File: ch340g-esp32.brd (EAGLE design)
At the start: 100 x 80 mm, 0 parts

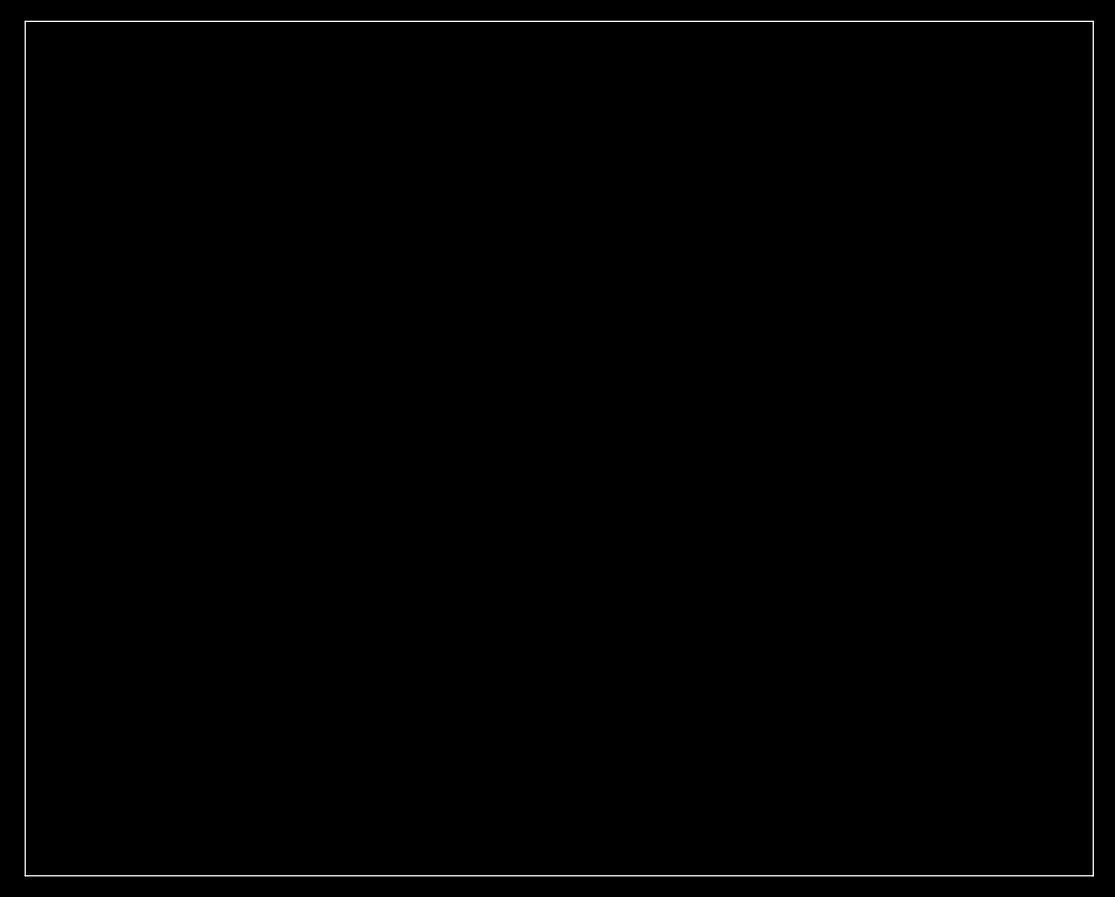
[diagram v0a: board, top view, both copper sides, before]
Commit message: rev1
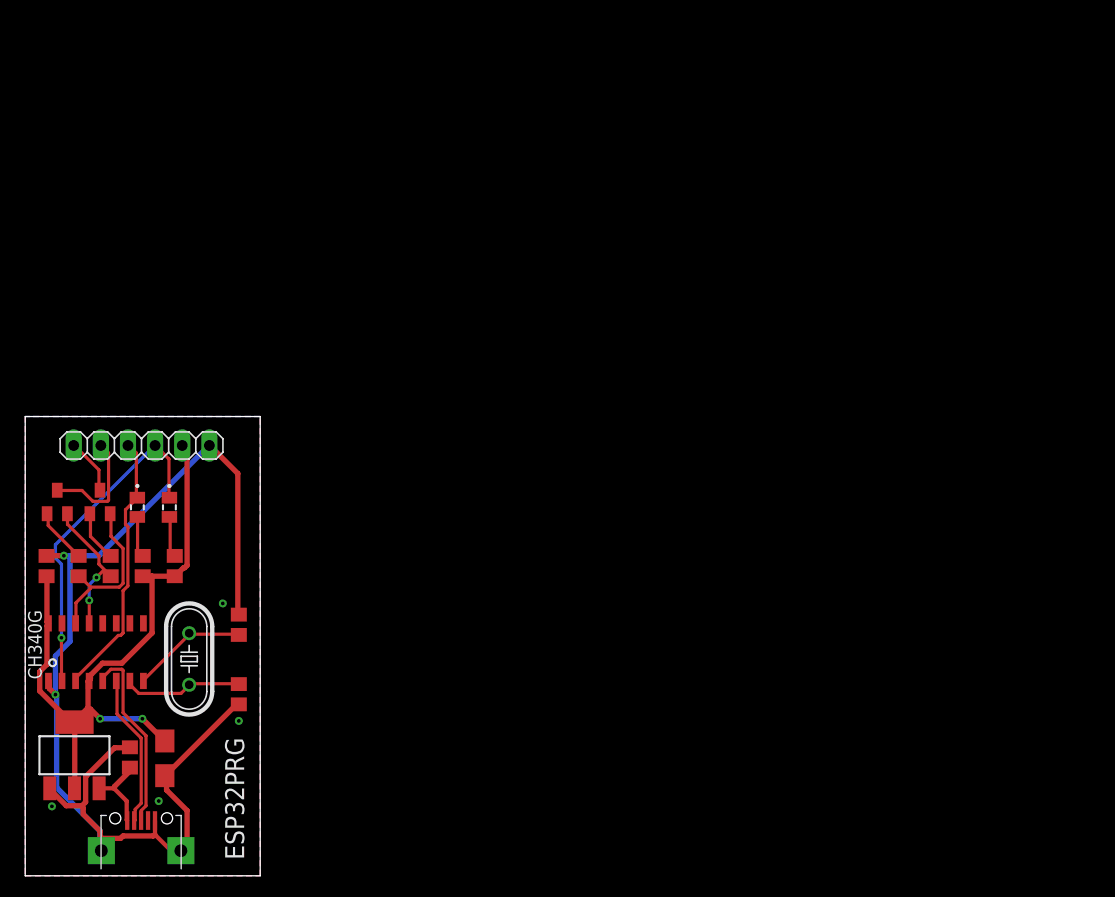
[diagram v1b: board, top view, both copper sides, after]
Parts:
- added C1, C2: 22, rcl:C0805
- added C3, C5: 0.1uF, rcl:C0805
- added C4: 10uF, rcl:B/3528-21W
- added D1: YELLOW, 597-5311-402F:LEDC2012X70N
- added D2: GREEN, 597-5311-402F:LEDC2012X70N
- added IC1: (no value), lm1117:SOT223
- added JP1: OUT, pinhead:1X06
- added Q1: 12M, crystal:HC49/S
- added R1, R2: 10K, rcl:R0805
- added R3, R4: 2K, rcl:R0805
- added T1, T2: BC847, transistor:SOT23
- added U$1: MICRO-USB, microusb:MICRO-USB
- added U$2: CH340G, ch340g:SOIC16
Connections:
- new net +5V: C3.1, IC1.3, U$1.1
- new net D+: U$1.3, U$2.5
- new net D-: U$1.2, U$2.6
- new net DTR: R1.1, T2.2, U$2.13
- new net EN: JP1.1, T1.3
- new net GND: C1.2, C2.2, C3.2, C4.-, C5.2, IC1.1, JP1.6, U$1.5, U$1.GND1, U$1.GND2, U$2.1
- new net IO0: JP1.2, T2.3
- new net N$1: C2.1, Q1.2, U$2.8
- new net N$12: D2.A, R4.1
- new net N$2: C1.1, Q1.1, U$2.7
- new net N$3: R1.2, T1.1
- new net N$4: R2.2, T2.1
- new net N$5: D1.A, R3.1
- new net RTS: R2.1, T1.2, U$2.14
- new net RX: D2.C, JP1.3, U$2.3
- new net TX: D1.C, JP1.4, U$2.2
- new net VCC: C4.+, C5.1, IC1.2, IC1.TAB, JP1.5, R3.2, R4.2, U$2.16, U$2.4
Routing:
- net GND: track 0.00 -> 113.3 mm, vias 0 -> 6
- net VCC: track 0.00 -> 64.0 mm, vias 0 -> 2
- net TX: track 0.00 -> 31.7 mm, vias 0 -> 1
- net RX: track 0.00 -> 25.2 mm
- net D+: track 0.00 -> 17.7 mm
- net RTS: track 0.00 -> 15.7 mm
- net D-: track 0.00 -> 14.4 mm
- net DTR: track 0.00 -> 13.9 mm, vias 0 -> 2
- net N$2: track 0.00 -> 11.3 mm
- net N$1: track 0.00 -> 10.9 mm
- net IO0: track 0.00 -> 10.7 mm
- net +5V: track 0.00 -> 7.46 mm
- net EN: track 0.00 -> 5.25 mm
- net N$4: track 0.00 -> 5.18 mm
- net N$3: track 0.00 -> 4.78 mm
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- added copper zone on layer 1, net GND
- added copper zone on layer 16, net GND
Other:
- board size 100 x 80 mm -> 22 x 43 mm
- board text added: "ESP32PRG"
- board text added: "RST BOOT RX TX 3.3V GND"

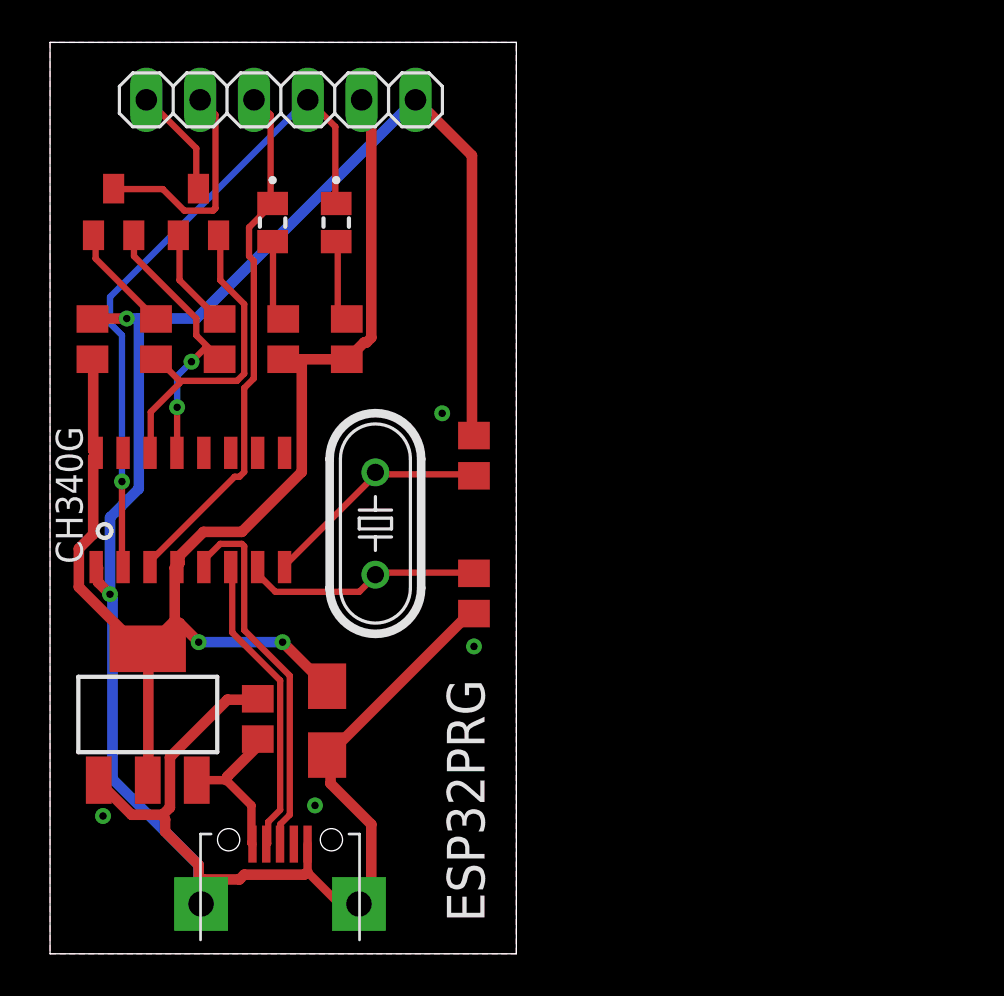
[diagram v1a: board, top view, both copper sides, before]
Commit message: board update
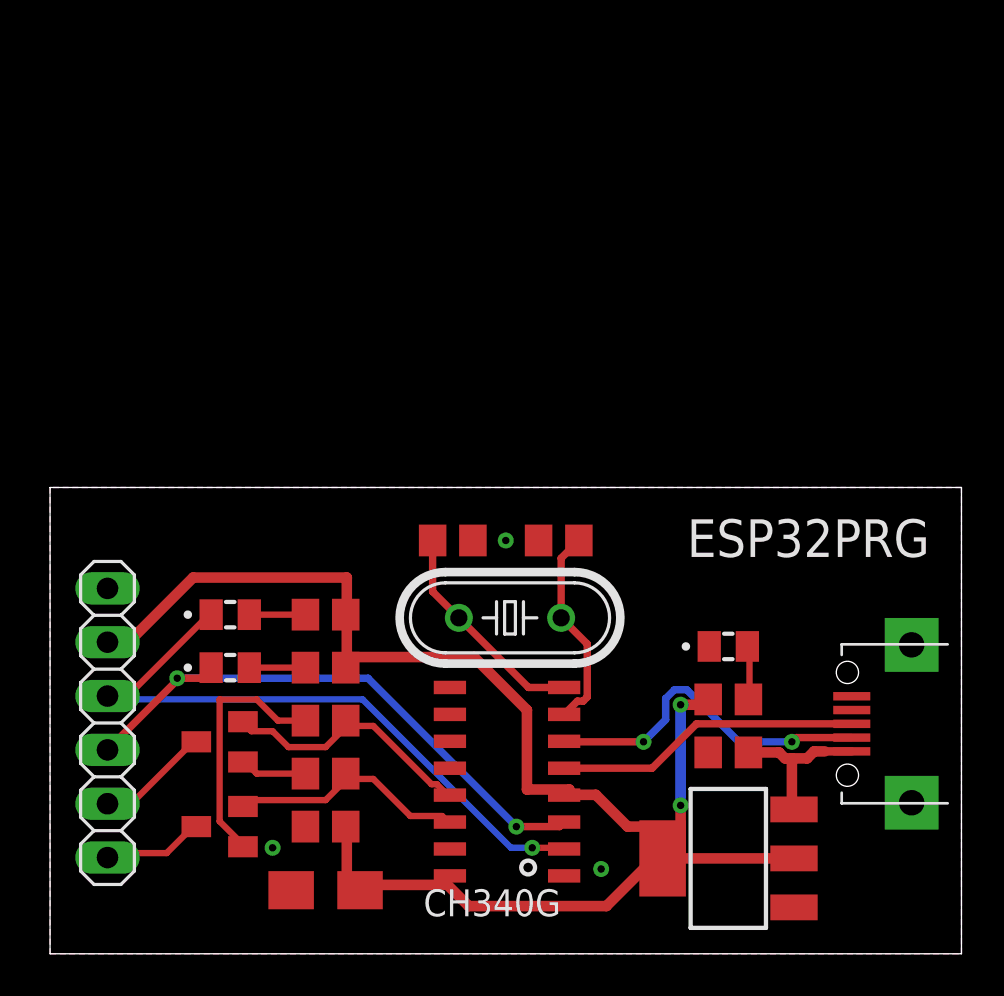
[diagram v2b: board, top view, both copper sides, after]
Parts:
- added D3: GREEN, 597-5311-402F:LEDC2012X70N
- added R5: 2K, rcl:R0805
- moved U$1 33.1 mm to (42.4, 10.8), turned to 90 degrees
- moved JP1 30.5 mm to (2.71, 10.9), turned to 90 degrees
- moved T1 29.0 mm to (8.00, 6.00), turned to 90 degrees
- moved IC1 28.2 mm to (32.0, 4.50), turned to 90 degrees
- moved C5 25.5 mm to (13.0, 6.00), turned to 180 degrees
- moved T2 25.5 mm to (8.00, 10.0), turned to 90 degrees
- moved C3 22.3 mm to (32.0, 9.50), turned to 180 degrees
- moved R2 22.0 mm to (13.0, 8.50), turned to 180 degrees
- moved D2 21.1 mm to (8.50, 13.5), turned to 0 degrees
- moved U$2 19.7 mm to (21.6, 8.12), turned to 90 degrees
- moved D1 19.2 mm to (8.50, 16.0), turned to 0 degrees
- moved R1 18.7 mm to (13.0, 11.0), turned to 180 degrees
- moved R4 15.6 mm to (13.0, 13.5), turned to 0 degrees
- moved R3 13.0 mm to (13.0, 16.0), turned to 0 degrees
- moved C4 8.00 mm to (13.0, 3.00), turned to 0 degrees
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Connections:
- new net N$6: D3.A, R5.1
- net GND: now also D3.C
- net VCC: now also R5.2
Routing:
- net GND: track 113.3 -> 0.00 mm, vias 6 -> 3
- net VCC: track 64.0 -> 76.0 mm
- net N$3: track 4.78 -> 11.9 mm
- net IO0: track 10.7 -> 5.46 mm
- net RTS: track 15.7 -> 12.0 mm
- net D+: track 17.7 -> 14.4 mm
- net N$6: track 0.00 -> 2.65 mm
- net RX: track 25.2 -> 27.8 mm, vias 0 -> 2
- net N$4: track 5.18 -> 3.17 mm
- net D-: track 14.4 -> 16.3 mm, vias 0 -> 2
- net N$2: track 11.3 -> 9.67 mm
- net N$5: track 3.92 -> 2.65 mm
- net N$12: track 3.86 -> 2.65 mm
- net DTR: track 13.9 -> 13.0 mm, vias 2 -> 0
- net TX: track 31.7 -> 31.1 mm
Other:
- board size 22 x 43 mm -> 43 x 22 mm
